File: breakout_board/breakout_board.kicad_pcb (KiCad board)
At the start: 2 copper layers, 60.7 x 33.3 mm, 2 parts, among them J1 Edge Connector, J2 Pin Header

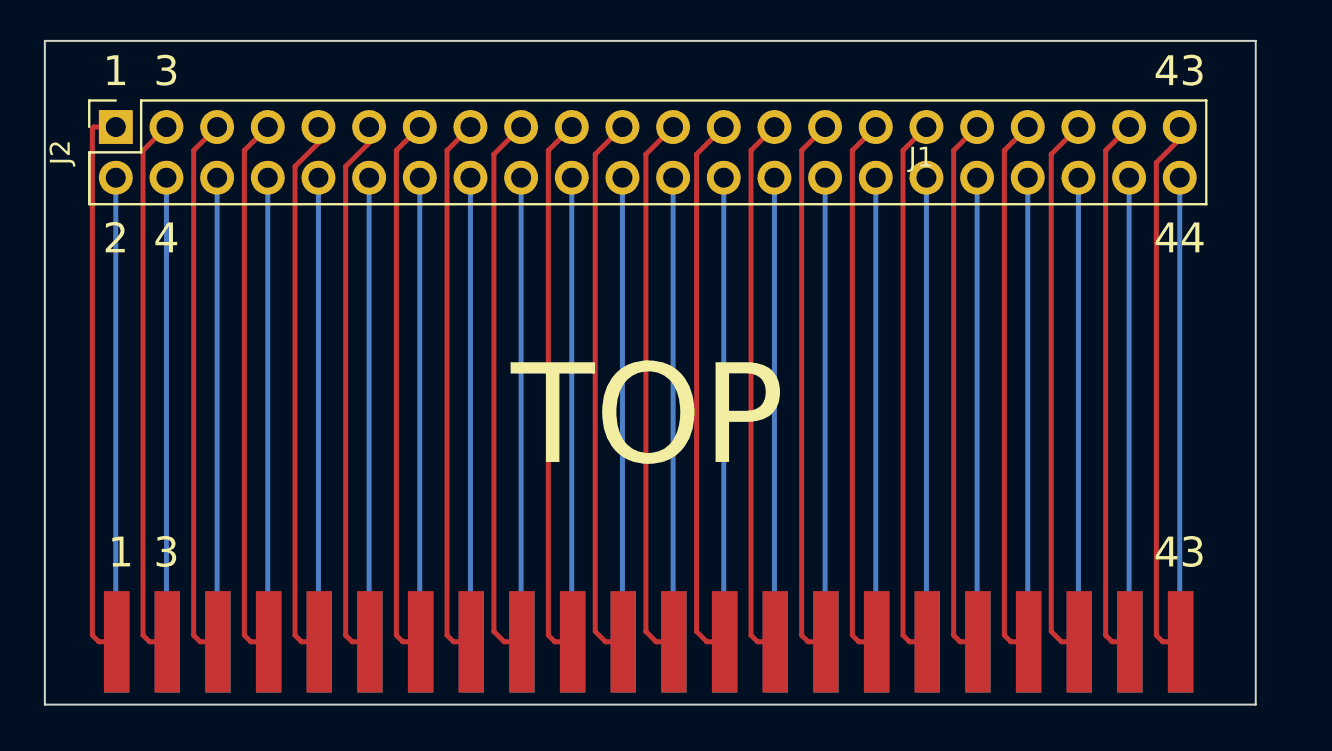
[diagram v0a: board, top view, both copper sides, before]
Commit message: Save progress on PCB.
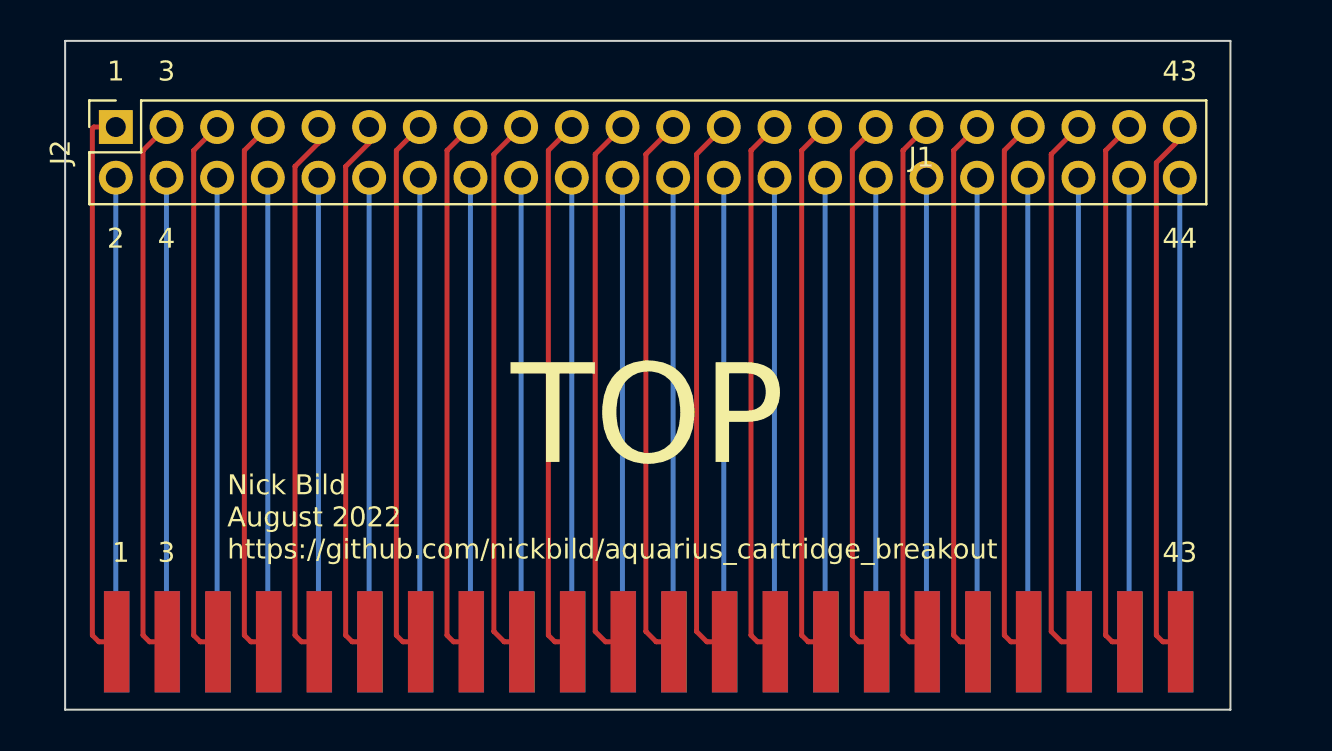
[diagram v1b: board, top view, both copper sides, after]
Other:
- board size 60.7 x 33.3 mm -> 58.4 x 33.5 mm
- board text added: "Nick Bild August 2022 https://github.com/nickbild/aquarius_cartridge_breakout"
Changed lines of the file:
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@@
   (general
     (thickness 1.6)
-    (drawings 17)
+    (drawings 18)
     (tracks 136)
     (zones 0)
@@
     (pad 43 connect rect (at 41.6941 12.0904) (size 1.27 5.08) (layers F.Cu F.Mask)
       (net 22 "Net-(J1-Pad43)"))
-    (pad 2 connect rect (at -11.63574 12.09294) (size 1.27 5.08) (layers B.Cu F.Mask)
+    (pad 2 connect rect (at -11.63574 12.09294) (size 1.27 5.08) (layers B.Cu B.Mask)
       (net 23 "Net-(J1-Pad2)"))
-    (pad 4 connect rect (at -9.09574 12.09294) (size 1.27 5.08) (layers B.Cu F.Mask)
+    (pad 4 connect rect (at -9.09574 12.09294) (size 1.27 5.08) (layers B.Cu B.Mask)
       (net 24 "Net-(J1-Pad4)"))
-    (pad 6 connect rect (at -6.55574 12.09294) (size 1.27 5.08) (layers B.Cu F.Mask)
+    (pad 6 connect rect (at -6.55574 12.09294) (size 1.27 5.08) (layers B.Cu B.Mask)
       (net 25 "Net-(J1-Pad6)"))
-    (pad 8 connect rect (at -4.01574 12.09294) (size 1.27 5.08) (layers B.Cu F.Mask)
+    (pad 8 connect rect (at -4.01574 12.09294) (size 1.27 5.08) (layers B.Cu B.Mask)
       (net 26 "Net-(J1-Pad8)"))
-    (pad 10 connect rect (at -1.47574 12.09294) (size 1.27 5.08) (layers B.Cu F.Mask)
+    (pad 10 connect rect (at -1.47574 12.09294) (size 1.27 5.08) (layers B.Cu B.Mask)
       (net 27 "Net-(J1-Pad10)"))
-    (pad 12 connect rect (at 1.06426 12.09294) (size 1.27 5.08) (layers B.Cu F.Mask)
+    (pad 12 connect rect (at 1.06426 12.09294) (size 1.27 5.08) (layers B.Cu B.Mask)
       (net 28 "Net-(J1-Pad12)"))
-    (pad 14 connect rect (at 3.60426 12.09294) (size 1.27 5.08) (layers B.Cu F.Mask)
+    (pad 14 connect rect (at 3.60426 12.09294) (size 1.27 5.08) (layers B.Cu B.Mask)
       (net 29 "Net-(J1-Pad14)"))
-    (pad 16 connect rect (at 6.14426 12.09294) (size 1.27 5.08) (layers B.Cu F.Mask)
+    (pad 16 connect rect (at 6.14426 12.09294) (size 1.27 5.08) (layers B.Cu B.Mask)
       (net 30 "Net-(J1-Pad16)"))
-    (pad 18 connect rect (at 8.68426 12.09294) (size 1.27 5.08) (layers B.Cu F.Mask)
+    (pad 18 connect rect (at 8.68426 12.09294) (size 1.27 5.08) (layers B.Cu B.Mask)
       (net 31 "Net-(J1-Pad18)"))
-    (pad 20 connect rect (at 11.22426 12.09294) (size 1.27 5.08) (layers B.Cu F.Mask)
+    (pad 20 connect rect (at 11.22426 12.09294) (size 1.27 5.08) (layers B.Cu B.Mask)
       (net 32 "Net-(J1-Pad20)"))
-    (pad 22 connect rect (at 13.76426 12.09294) (size 1.27 5.08) (layers B.Cu F.Mask)
+    (pad 22 connect rect (at 13.76426 12.09294) (size 1.27 5.08) (layers B.Cu B.Mask)
       (net 33 "Net-(J1-Pad22)"))
-    (pad 24 connect rect (at 16.30426 12.09294) (size 1.27 5.08) (layers B.Cu F.Mask)
+    (pad 24 connect rect (at 16.30426 12.09294) (size 1.27 5.08) (layers B.Cu B.Mask)
       (net 34 "Net-(J1-Pad24)"))
-    (pad 26 connect rect (at 18.84426 12.09294) (size 1.27 5.08) (layers B.Cu F.Mask)
+    (pad 26 connect rect (at 18.84426 12.09294) (size 1.27 5.08) (layers B.Cu B.Mask)
       (net 35 "Net-(J1-Pad26)"))
-    (pad 28 connect rect (at 21.38426 12.09294) (size 1.27 5.08) (layers B.Cu F.Mask)
+    (pad 28 connect rect (at 21.38426 12.09294) (size 1.27 5.08) (layers B.Cu B.Mask)
       (net 36 "Net-(J1-Pad28)"))
-    (pad 30 connect rect (at 23.92426 12.09294) (size 1.27 5.08) (layers B.Cu F.Mask)
+    (pad 30 connect rect (at 23.92426 12.09294) (size 1.27 5.08) (layers B.Cu B.Mask)
       (net 37 "Net-(J1-Pad30)"))
-    (pad 32 connect rect (at 26.46426 12.09294) (size 1.27 5.08) (layers B.Cu F.Mask)
+    (pad 32 connect rect (at 26.46426 12.09294) (size 1.27 5.08) (layers B.Cu B.Mask)
       (net 38 "Net-(J1-Pad32)"))
-    (pad 34 connect rect (at 29.00426 12.09294) (size 1.27 5.08) (layers B.Cu F.Mask)
+    (pad 34 connect rect (at 29.00426 12.09294) (size 1.27 5.08) (layers B.Cu B.Mask)
       (net 39 "Net-(J1-Pad34)"))
-    (pad 36 connect rect (at 31.54426 12.09294) (size 1.27 5.08) (layers B.Cu F.Mask)
+    (pad 36 connect rect (at 31.54426 12.09294) (size 1.27 5.08) (layers B.Cu B.Mask)
       (net 40 "Net-(J1-Pad36)"))
-    (pad 38 connect rect (at 34.08426 12.09294) (size 1.27 5.08) (layers B.Cu F.Mask)
+    (pad 38 connect rect (at 34.08426 12.09294) (size 1.27 5.08) (layers B.Cu B.Mask)
       (net 41 "Net-(J1-Pad38)"))
-    (pad 40 connect rect (at 36.62426 12.09294) (size 1.27 5.08) (layers B.Cu F.Mask)
+    (pad 40 connect rect (at 36.62426 12.09294) (size 1.27 5.08) (layers B.Cu B.Mask)
       (net 42 "Net-(J1-Pad40)"))
-    (pad 42 connect rect (at 39.16426 12.09294) (size 1.27 5.08) (layers B.Cu F.Mask)
+    (pad 42 connect rect (at 39.16426 12.09294) (size 1.27 5.08) (layers B.Cu B.Mask)
       (net 43 "Net-(J1-Pad42)"))
-    (pad 44 connect rect (at 41.70426 12.09294) (size 1.27 5.08) (layers B.Cu F.Mask)
+    (pad 44 connect rect (at 41.70426 12.09294) (size 1.27 5.08) (layers B.Cu B.Mask)
       (net 44 "Net-(J1-Pad44)"))
   )
@@
     )
   )
-  (gr_line (start 189.738 84.328) (end 189.738 117.602) (layer Edge.Cuts) (width 0.1))
-  (gr_line (start 129.032 84.328) (end 189.738 84.328) (layer Edge.Cuts) (width 0.1))
-  (gr_line (start 129.032 117.602) (end 129.032 84.328) (layer Edge.Cuts) (width 0.1))
-  (gr_line (start 189.738 117.602) (end 129.032 117.602) (layer Edge.Cuts) (width 0.1))
+  (gr_text "Nick Bild\nAugust 2022\nhttps://github.com/nickbild/aquarius_cartridge_breakout" (at 138.176 108.204) (layer F.SilkS)
+    (effects (font (size 1 1) (thickness 0.15)) (justify left))
+  )
+  (gr_line (start 188.468 84.328) (end 188.468 117.856) (layer Edge.Cuts) (width 0.1))
+  (gr_line (start 130.048 84.328) (end 188.468 84.328) (layer Edge.Cuts) (width 0.1))
+  (gr_line (start 130.048 117.856) (end 130.048 84.328) (layer Edge.Cuts) (width 0.1))
+  (gr_line (start 188.468 117.856) (end 130.048 117.856) (layer Edge.Cuts) (width 0.1))
   (gr_text 44 (at 185.928 110.49) (layer B.SilkS)
-    (effects (font (size 1.5 1.5) (thickness 0.3)))
+    (effects (font (size 1 1) (thickness 0.2)) (justify mirror))
   )
   (gr_text 4 (at 135.128 110.236) (layer B.SilkS)
-    (effects (font (size 1.5 1.5) (thickness 0.3)))
+    (effects (font (size 1 1) (thickness 0.2)) (justify mirror))
   )
   (gr_text 2 (at 132.588 110.236) (layer B.SilkS)
-    (effects (font (size 1.5 1.5) (thickness 0.3)))
+    (effects (font (size 1 1) (thickness 0.2)) (justify mirror))
   )
   (gr_text 44 (at 185.928 94.234) (layer F.SilkS)
-    (effects (font (size 1.5 1.5) (thickness 0.3)))
+    (effects (font (size 1 1) (thickness 0.2)))
   )
   (gr_text 4 (at 135.128 94.234) (layer F.SilkS)
-    (effects (font (size 1.5 1.5) (thickness 0.3)))
+    (effects (font (size 1 1) (thickness 0.2)))
   )
   (gr_text 2 (at 132.588 94.234) (layer F.SilkS)
-    (effects (font (size 1.5 1.5) (thickness 0.3)))
+    (effects (font (size 1 1) (thickness 0.2)))
   )
   (gr_text 43 (at 185.928 85.852) (layer F.SilkS)
-    (effects (font (size 1.5 1.5) (thickness 0.3)))
+    (effects (font (size 1 1) (thickness 0.2)))
   )
   (gr_text 3 (at 135.128 85.852) (layer F.SilkS)
-    (effects (font (size 1.5 1.5) (thickness 0.3)))
+    (effects (font (size 1 1) (thickness 0.2)))
   )
   (gr_text 1 (at 132.588 85.852) (layer F.SilkS)
-    (effects (font (size 1.5 1.5) (thickness 0.3)))
+    (effects (font (size 1 1) (thickness 0.2)))
   )
   (gr_text 43 (at 185.928 109.982) (layer F.SilkS)
-    (effects (font (size 1.5 1.5) (thickness 0.3)))
+    (effects (font (size 1 1) (thickness 0.2)))
   )
   (gr_text 3 (at 135.128 109.982) (layer F.SilkS)
-    (effects (font (size 1.5 1.5) (thickness 0.3)))
+    (effects (font (size 1 1) (thickness 0.2)))
   )
   (gr_text 1 (at 132.842 109.982) (layer F.SilkS)
-    (effects (font (size 1.5 1.5) (thickness 0.3)))
+    (effects (font (size 1 1) (thickness 0.2)))
   )
   (gr_text TOP (at 159.258 103.124) (layer F.SilkS)
